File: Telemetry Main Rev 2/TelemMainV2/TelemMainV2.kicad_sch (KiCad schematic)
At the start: 21 parts, among them J1 8 pin ATM connector, J3 12 pin ATM connector, J4 SD to SPI (Molex nanofit), U3 NUCLEO-F446RE, U4 ISO1050DUB, U6 MCP6004, U8 ISO1050DUB

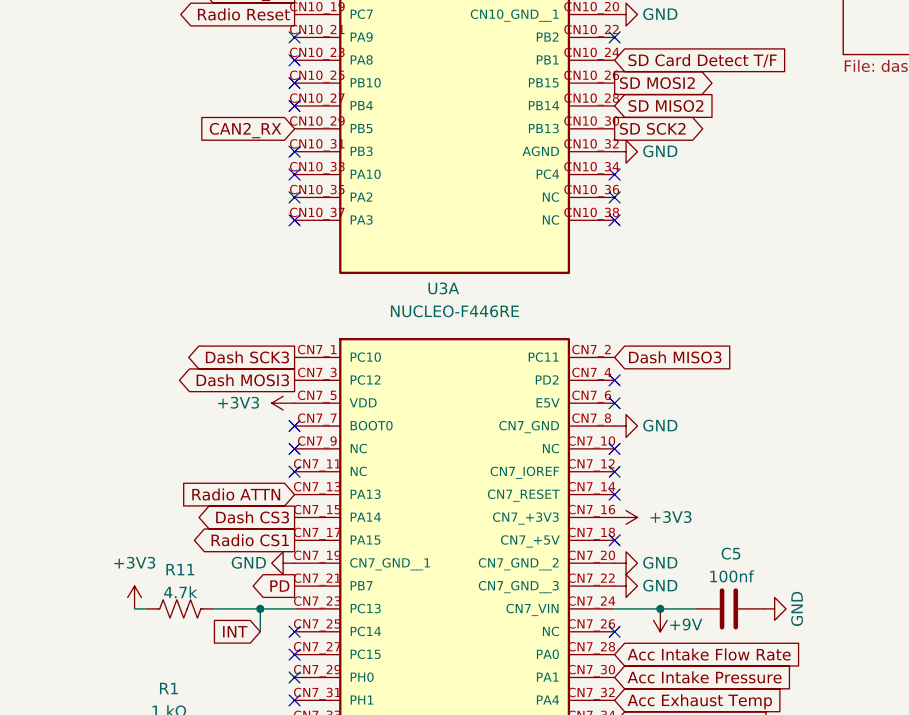
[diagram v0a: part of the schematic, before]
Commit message: updated dash traces
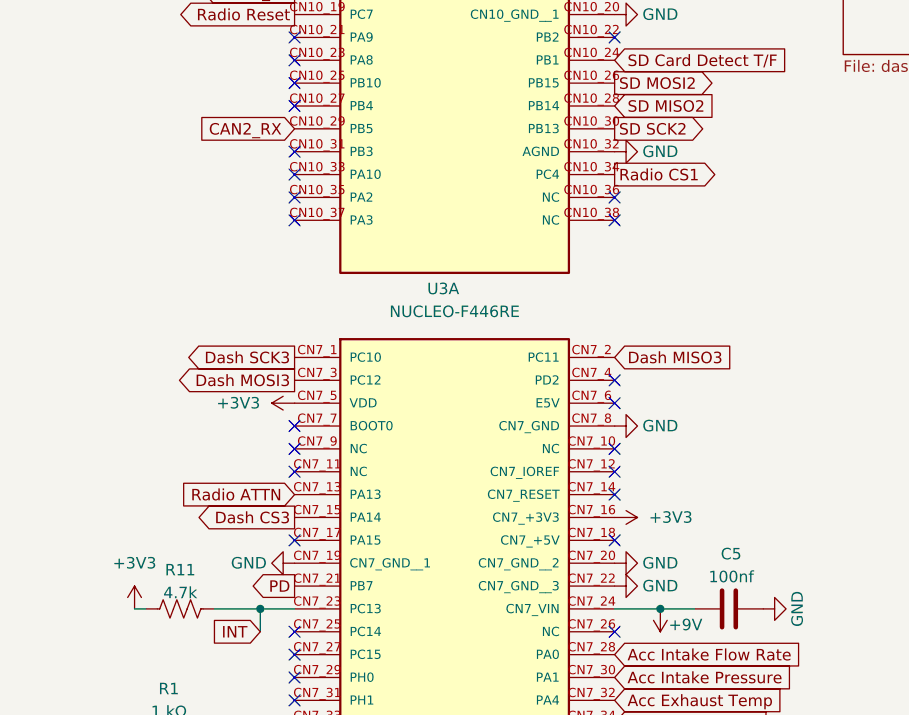
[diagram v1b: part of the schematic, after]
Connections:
- net Radio CS1: now also U3.CN10_34 (PC4); no longer U3.CN7_17 (PA15)
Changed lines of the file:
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@@
-	)
-	(no_connect
-		(at 201.93 60.96)
 	)
 	(no_connect
@@
 	(no_connect
 		(at 201.93 91.44)
+	)
+	(no_connect
+		(at 166.37 101.6)
 	)
 	(no_connect
@@
 		)
 	)
+	(global_label "Radio CS1"
+		(shape output)
+		(at 201.93 60.96 0)
+		(fields_autoplaced yes)
+		(effects
+			(font
+				(size 1.27 1.27)
+			)
+			(justify left)
+		)
+		(property "Intersheetrefs" "${INTERSHEET_REFS}"
+			(at 214.8936 60.96 0)
+			(effects
+				(font
+					(size 1.27 1.27)
+				)
+				(justify left)
+				(hide yes)
+			)
+		)
+	)
 	(global_label "Acc Intake Temp"
 		(shape output)
@@
 				(hide yes)
 			)
-		)
-	)
-	(global_label "Radio CS1"
-		(shape output)
-		(at 166.37 101.6 180)
-		(fields_autoplaced yes)
-		(effects
-			(font
-				(size 1.27 1.27)
-			)
-			(justify right)
-		)
-		(property "Intersheetrefs" "${INTERSHEET_REFS}"
-			(at 153.4064 101.6 0)
-			(effects
-				(font
-					(size 1.27 1.27)
-				)
-				(justify right)
-				(hide yes)
-			)

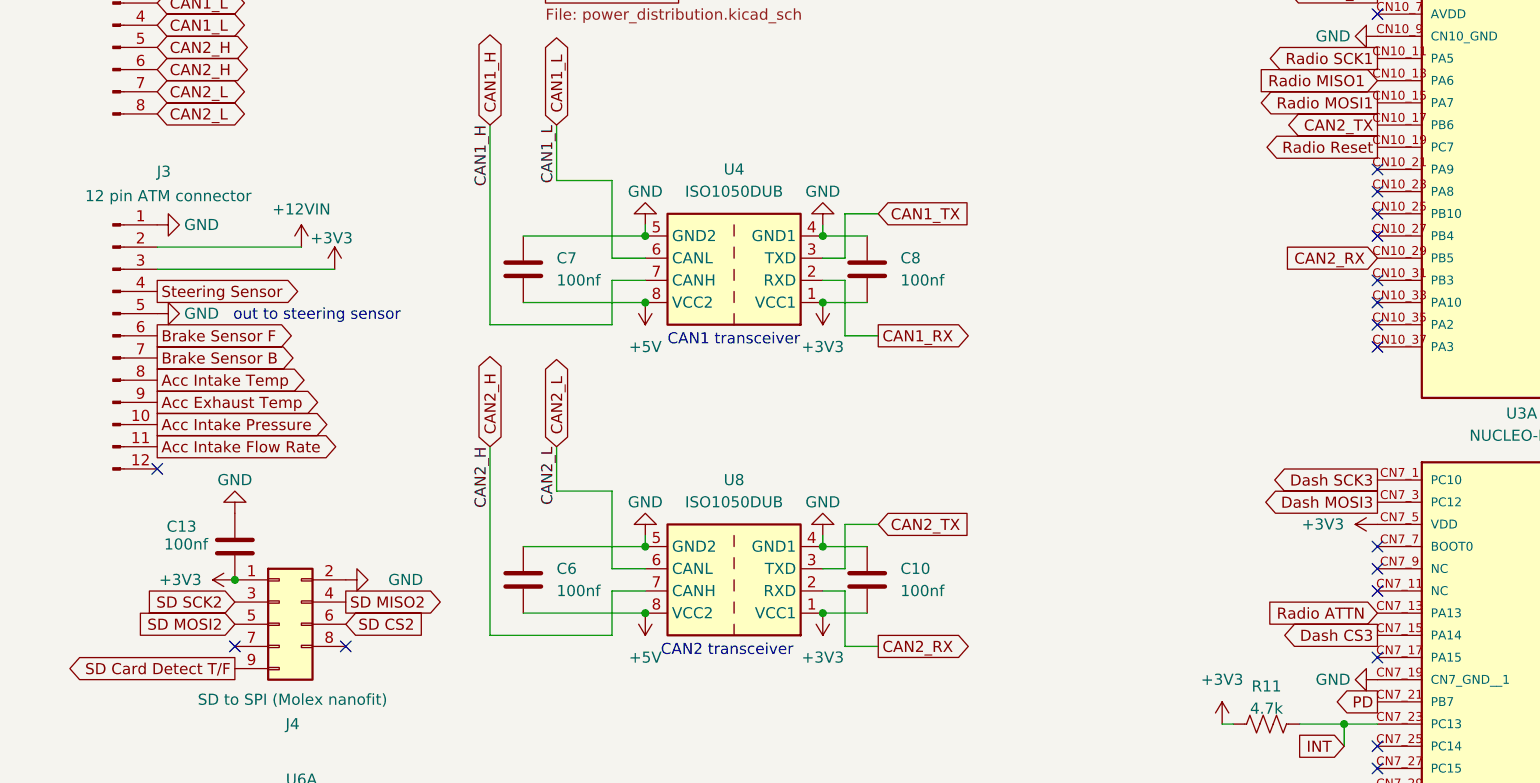
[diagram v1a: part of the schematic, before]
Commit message: almost done with dash traces
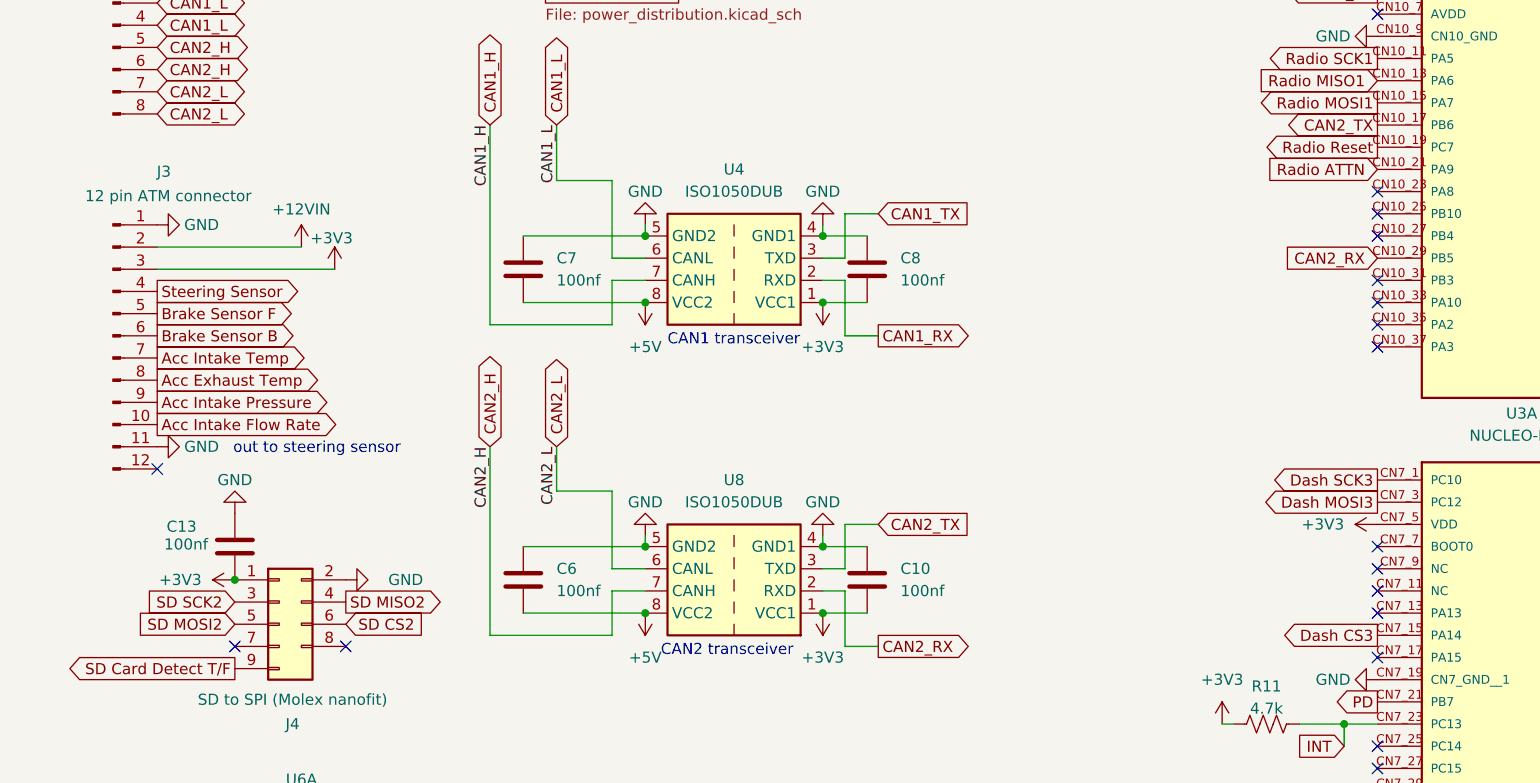
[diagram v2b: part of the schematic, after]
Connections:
- net Acc Exhaust Temp: now also J3.8 (Pin_8); no longer J3.9 (Pin_9)
- net Acc Intake Flow Rate: now also J3.10 (Pin_10); no longer J3.11 (Pin_11)
- net Acc Intake Pressure: now also J3.9 (Pin_9); no longer J3.10 (Pin_10)
- net Acc Intake Temp: now also J3.7 (Pin_7); no longer J3.8 (Pin_8)
- net Brake Sensor B: now also J3.6 (Pin_6); no longer J3.7 (Pin_7)
- net Brake Sensor F: now also J3.5 (Pin_5); no longer J3.6 (Pin_6)
- net GND: now also J3.11 (Pin_11); no longer J3.5 (Pin_5)
- net Radio ATTN: now also U3.CN10_21 (PA9); no longer U3.CN7_13 (PA13)
